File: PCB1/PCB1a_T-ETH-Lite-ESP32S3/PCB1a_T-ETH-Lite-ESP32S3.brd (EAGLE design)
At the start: 125.6 x 84.2 mm, 28 parts, among them J1 691357310006B, J2 618009231421, J5 61004021821, J6 61004021821, U2 MAX232D, U4 TLE9250VSJ, U8 74AHCT245, U9 74AHCT245

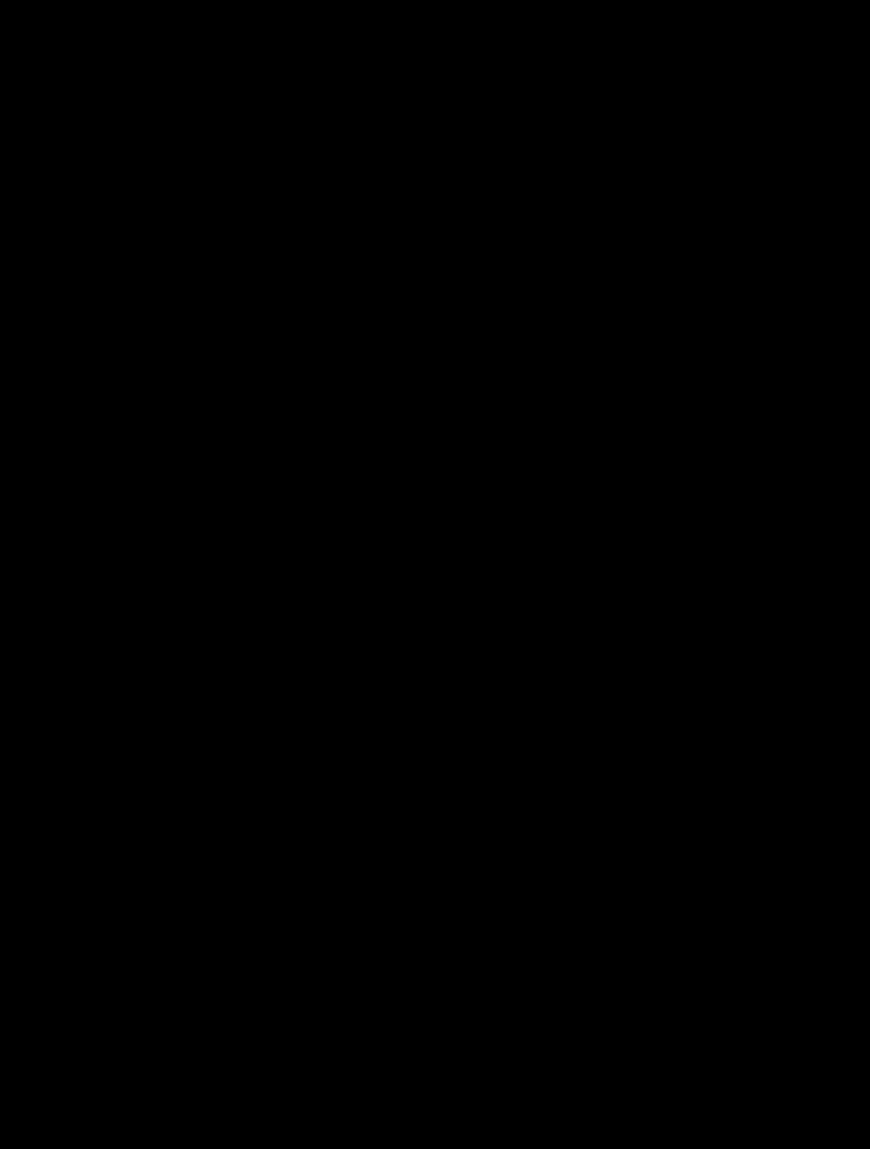
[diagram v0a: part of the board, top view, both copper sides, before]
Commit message: ..
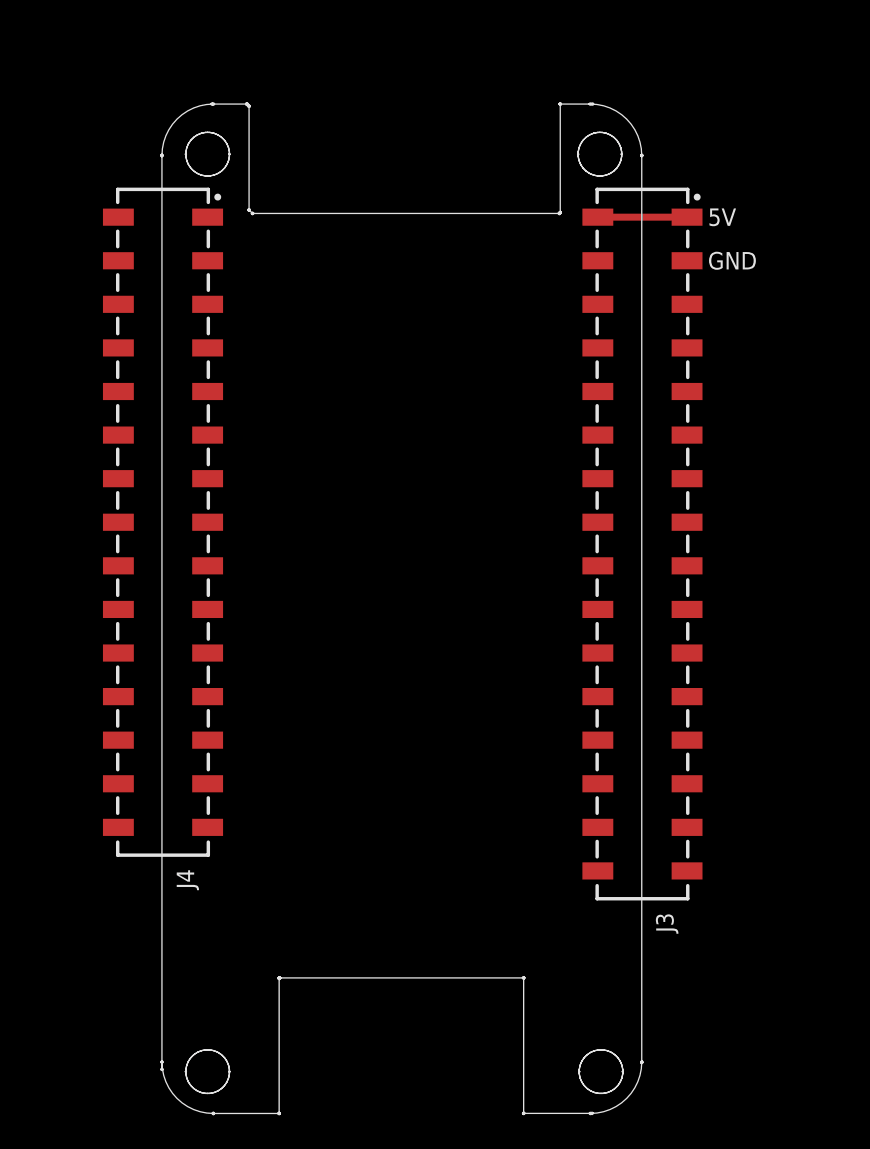
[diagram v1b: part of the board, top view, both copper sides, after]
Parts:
- added J3: 61003221821, Wurth_Connectors_WR-PHD:61003221821
- added J4: 61003021821, Wurth_Connectors_WR-PHD:61003021821
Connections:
- net +5V: now also J3.1, J3.2
- net GND: now also J3.3, J3.4
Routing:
- net +5V: track 34.0 -> 39.2 mm
